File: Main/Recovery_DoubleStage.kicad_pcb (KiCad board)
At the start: 2 copper layers, 66 parts, among them IC1 ATMEGA2560-16AU, IC2 AP2210N-3.3TRG1, IC3 MMC5983MA, IC4 NEO-6M-0, IC5 BMP388, IC6 MPU-6050, J1 ICSP, J2 Conn_02x10_Counter_Clockwise, J3 Conn_Coaxial, J4 Conn_Coaxial, J5 MEM2075-00-140-01-A, J6 XT60PW-M, Q1 BSS138, SW1 SW_Push, U1 NCP5501DT50RKG, U2 RFM95W-868S2, Y1 CSTNE16M0V530000R0

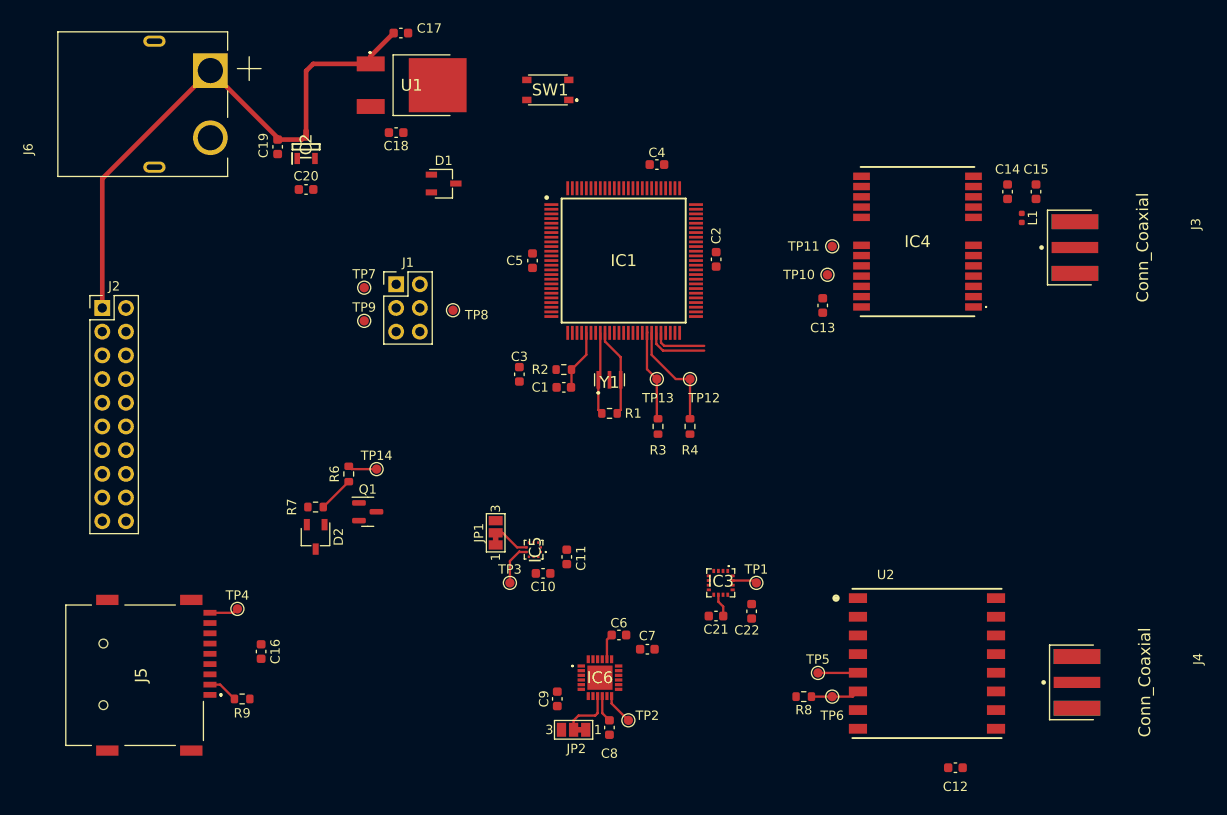
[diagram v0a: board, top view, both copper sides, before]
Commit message: almost done with routing
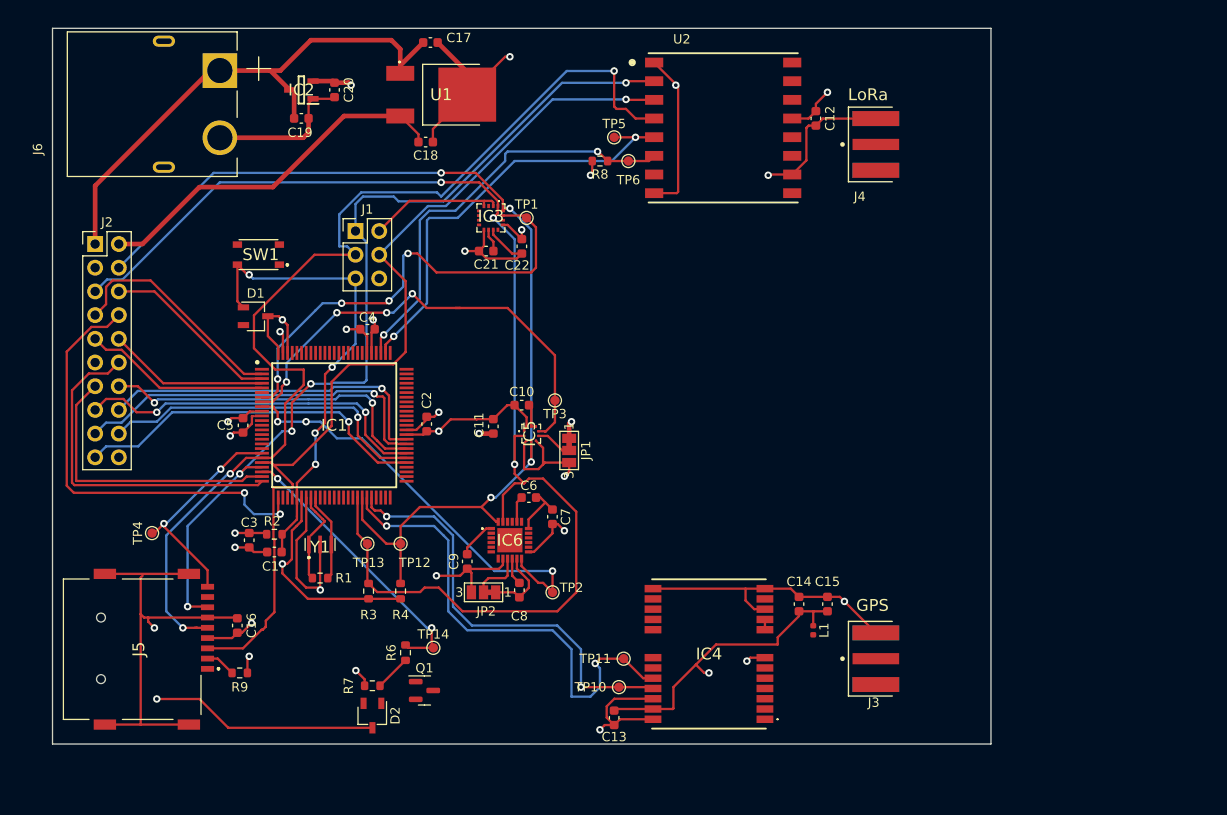
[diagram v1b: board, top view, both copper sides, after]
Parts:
- removed TP7: MISO, TestPoint:TestPoint_Pad_D1.0mm
- removed TP8: MOSI, TestPoint:TestPoint_Pad_D1.0mm
- removed TP9: SCK, TestPoint:TestPoint_Pad_D1.0mm
- J3: value Conn_Coaxial -> GPS
- J4: value Conn_Coaxial -> LoRa
- moved C12 71.2 mm to (94.3, 22.9), turned to -90 degrees
- moved J4 61.6 mm to (108.0, 25.7)
- moved TP5 61.4 mm to (72.6, 24.9)
- moved R8 61.4 mm to (71.1, 27.4)
- moved TP6 61.4 mm to (74.2, 27.4)
- moved U2 61.4 mm to (84.3, 23.9)
- moved C14 49.5 mm to (92.5, 74.9)
- moved IC4 49.5 mm to (82.8, 80.3)
- moved L1 49.5 mm to (94.0, 77.7)
- moved TP11 49.5 mm to (73.7, 80.8)
- moved C13 49.5 mm to (72.6, 87.1)
- moved C15 49.5 mm to (95.5, 74.9)
- moved TP10 49.5 mm to (73.2, 83.8)
- moved J3 49.0 mm to (108.0, 80.8)
- moved C21 46.2 mm to (58.9, 37.1)
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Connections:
- net Net-(IC4-Pad11) renamed /ANT_NEO
- net Net-(J4-Pad1) renamed /ANT_LORA
- IC1 pad 55: /ID3 -> /ID1
- IC1 pad 56: /IGNITION -> /ID2
- IC1 pad 57: /ID1 -> /ID3
- IC1 pad 58: /ID2 -> /IGNITION
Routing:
- net GND: track 0.00 -> 247.1 mm, vias 0 -> 17
- net +3V3: track 0.00 -> 187.0 mm, vias 0 -> 16
- net /SCL: track 9.84 -> 140.6 mm, vias 0 -> 3
- net +5V: track 0.00 -> 115.1 mm, vias 0 -> 1
- net /SCK: track 0.00 -> 112.9 mm, vias 0 -> 3
- net /SDA: track 11.8 -> 112.0 mm, vias 0 -> 4
- net /MOSI: track 0.00 -> 99.1 mm, vias 0 -> 1
- net /MISO: track 0.00 -> 98.2 mm, vias 0 -> 5
- net /OPT1: track 0.00 -> 48.3 mm, vias 0 -> 2
- net /MMC_INT: track 2.65 -> 49.8 mm, vias 0 -> 4
- net /BMP_INT: track 4.56 -> 50.4 mm, vias 0 -> 4
- net /RX1: track 6.62 -> 52.4 mm, vias 0 -> 2
- net /microcontroller/RESET: track 6.52 -> 50.8 mm, vias 0 -> 4
- net /MPU_INT: track 3.34 -> 46.8 mm, vias 0 -> 3
- net /LoRa_CS: track 4.29 -> 46.4 mm, vias 0 -> 2
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- added copper zone on In2.Cu, net +3V3
- added copper zone on In1.Cu, net GND
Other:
- board outline added: 100.6 x 76.7 mm
- copper layers 2 -> 4
